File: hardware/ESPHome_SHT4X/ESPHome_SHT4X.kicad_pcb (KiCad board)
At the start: 2 copper layers, 50 x 30.6 mm, 43 parts, among them J2 UJ20-C-H-G-SMT-2A-P16-TR, SW1 SW_Push, SW2 SW_Push, SW3 SW_Push, U1 ESP32-C6-WROOM-1-N8, U2 BQ25628ERYKR, U3 SHT40-AD1F-R2, U4 XC6220B331MR-G

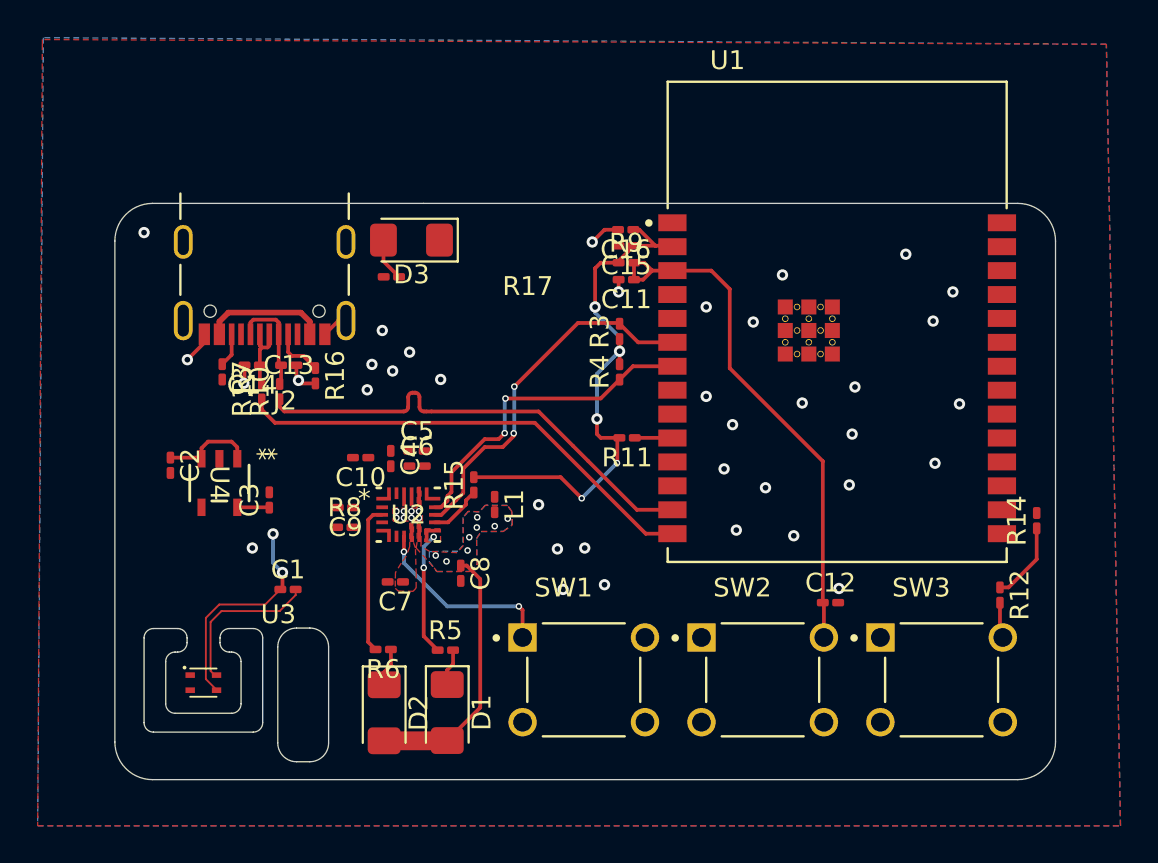
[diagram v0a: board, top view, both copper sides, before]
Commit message: Continued work on PCB Layout
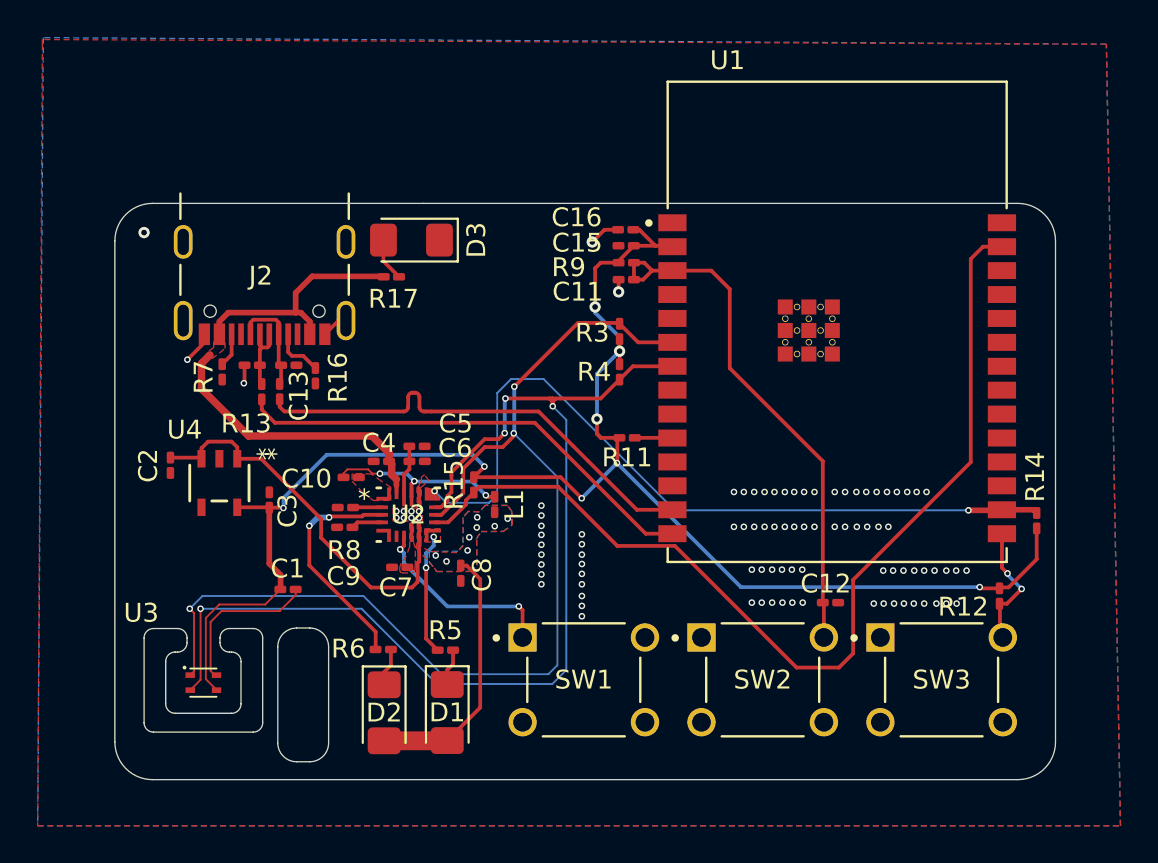
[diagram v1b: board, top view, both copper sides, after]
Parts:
- moved C10 1.16 mm to (142.4, 69.8), turned to 0 degrees
- moved C7 0.81 mm to (145.0, 74.5)
- moved C4 0.52 mm to (144.0, 68.9), turned to 180 degrees
- moved C5 0.25 mm to (145.9, 68.1)
- moved C6 0.25 mm to (145.9, 68.9)
- moved R12 0.06 mm to (176.8, 76.0)
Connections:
- U1 pad 19: IO19 -> IO21
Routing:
- net *INT: track 2.86 -> 52.9 mm
- net IO18: track 0.00 -> 42.2 mm, vias 0 -> 2
- net SCL: track 17.5 -> 59.2 mm, vias 2 -> 4
- net SDA: track 19.7 -> 58.4 mm, vias 2 -> 3
- net ESP_3V3: track 46.7 -> 85.3 mm, vias 7 -> 8
- net VBUS: track 6.54 -> 28.3 mm
- net SYS: track 19.0 -> 34.8 mm
- net SW: track 0.00 -> 9.76 mm, vias 0 -> 3
- net Net-(U1-IO9): track 1.90 -> 6.77 mm, vias 0 -> 2
- net Net-(U2-*PG): track 7.90 -> 12.1 mm, vias 0 -> 2
- net PMID: track 0.00 -> 2.80 mm
- net GND: track 16.8 -> 15.0 mm, vias 45 -> 95
- net ILIM: track 0.00 -> 1.69 mm
- net Net-(U2-REGN): track 0.00 -> 1.55 mm
- net IO21: track 0.00 -> 0.58 mm
- added copper zone on F.Cu, net BTST
- added copper zone on F.Cu, net VBUS
